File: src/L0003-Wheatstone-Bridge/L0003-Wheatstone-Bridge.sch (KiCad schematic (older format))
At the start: 18 parts, among them P1 12V, P2 2043-1X04G00DAU, U1 MCP1703T-4002E_DB

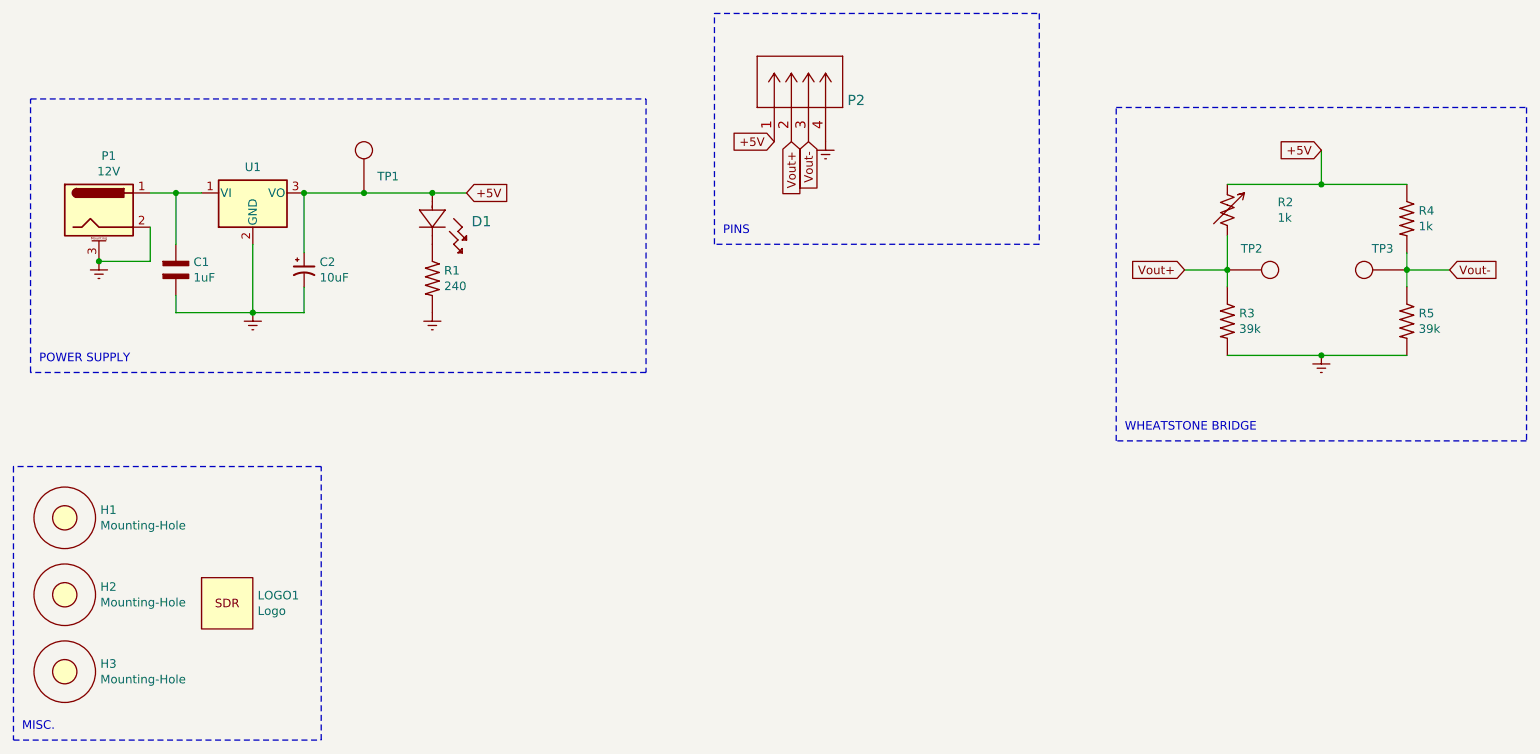
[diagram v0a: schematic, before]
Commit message: Created PCB Layout
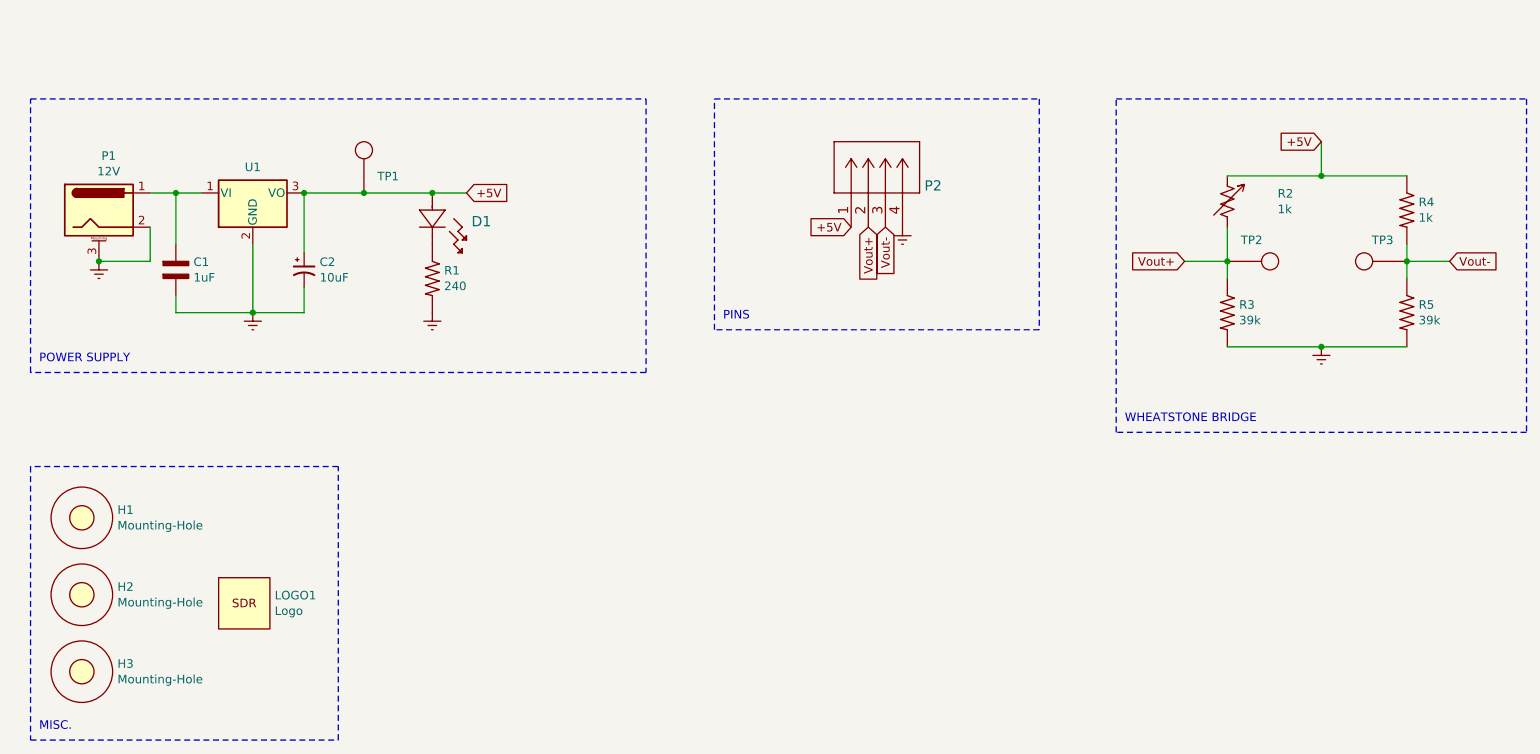
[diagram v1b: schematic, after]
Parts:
- C1: footprint (none) -> L0003-Wheatstone-Bridge:CAP_0603
- C2: footprint (none) -> L0003-Wheatstone-Bridge:T491A106K010AT
- D1: footprint (none) -> L0003-Wheatstone-Bridge:SML-LX1206GC-TR
- H1, H2, H3: footprint (none) -> L0003-Wheatstone-Bridge:MountingHole_2.1mm
- LOGO1: footprint (none) -> L0003-Wheatstone-Bridge:logo2
- P1: footprint (none) -> L0003-Wheatstone-Bridge:12V_power_jack
- P2: footprint CONN_2043-1X04G00DAU_OUP -> L0003-Wheatstone-Bridge:SULLINS_PPTC041LFBN-RC
- R1, R3, R4, R5: footprint (none) -> L0003-Wheatstone-Bridge:RES_0603
- R2: footprint (none) -> L0003-Wheatstone-Bridge:TRIM_3310Y-001-102L
- TP1, TP2, TP3: footprint (none) -> L0003-Wheatstone-Bridge:TP
- U1: footprint Package_TO_SOT_SMD:SOT-223-3_TabPin2 -> L0003-Wheatstone-Bridge:MCP1703T-4002E&slash_DB
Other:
- moved on the sheet: H1, H2, H3, LOGO1, P2, R2, R3, R4, R5

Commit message: Finished PCB
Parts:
- U1: footprint L0003-Wheatstone-Bridge:MCP1703T-4002E&slash_DB -> Package_TO_SOT_SMD:SOT-223-3_TabPin2
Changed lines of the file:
@@
 F 0 "U1" H 2100 2701 50  0000 C CNN
 F 1 "MCP1703T-4002E_DB" H 2100 2675 50  0001 L CNN
-F 2 "L0003-Wheatstone-Bridge:MCP1703T-4002E&slash_DB" H 2100 2750 50  0001 C CNN
+F 2 "Package_TO_SOT_SMD:SOT-223-3_TabPin2" H 2100 2750 50  0001 C CNN
 F 3 "" H 2100 2500 50  0001 C CNN
 	1    2100 2550
